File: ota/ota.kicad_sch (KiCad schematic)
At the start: 19 parts, among them J3 Conn_01x04_Pin, J4 Conn_01x04_Pin, Q1 BC856BDW1, Q2 BC846BDW1, Q3 BC846BDW1, Q4 BC856BDW1, Q5 BC846BDW1, Q8 BC846BDW1, Q9 BC856BDW1

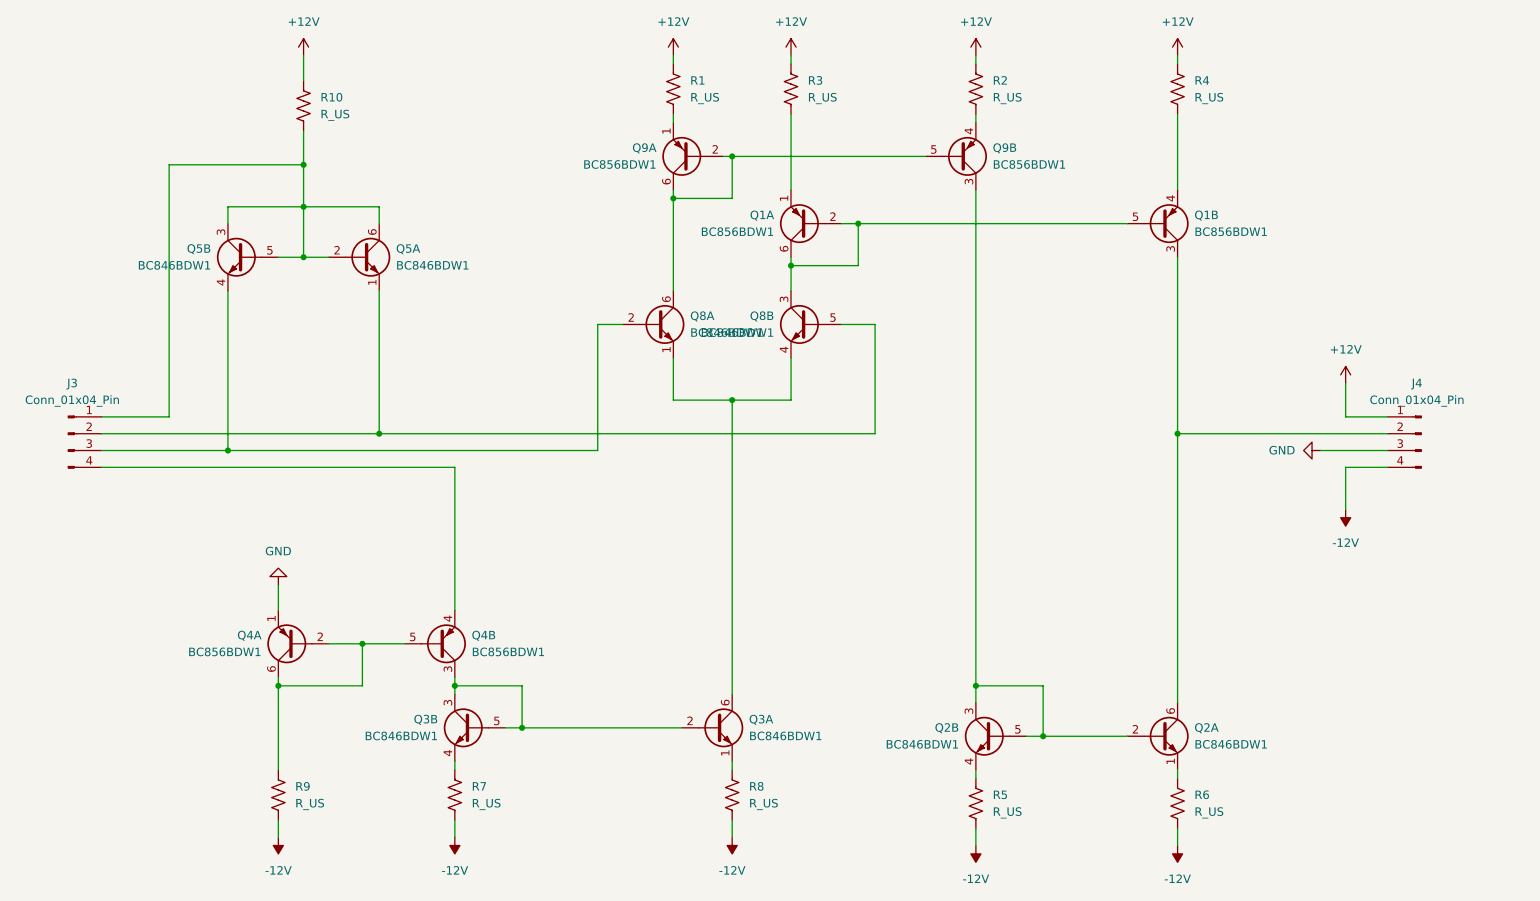
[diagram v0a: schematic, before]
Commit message: v1
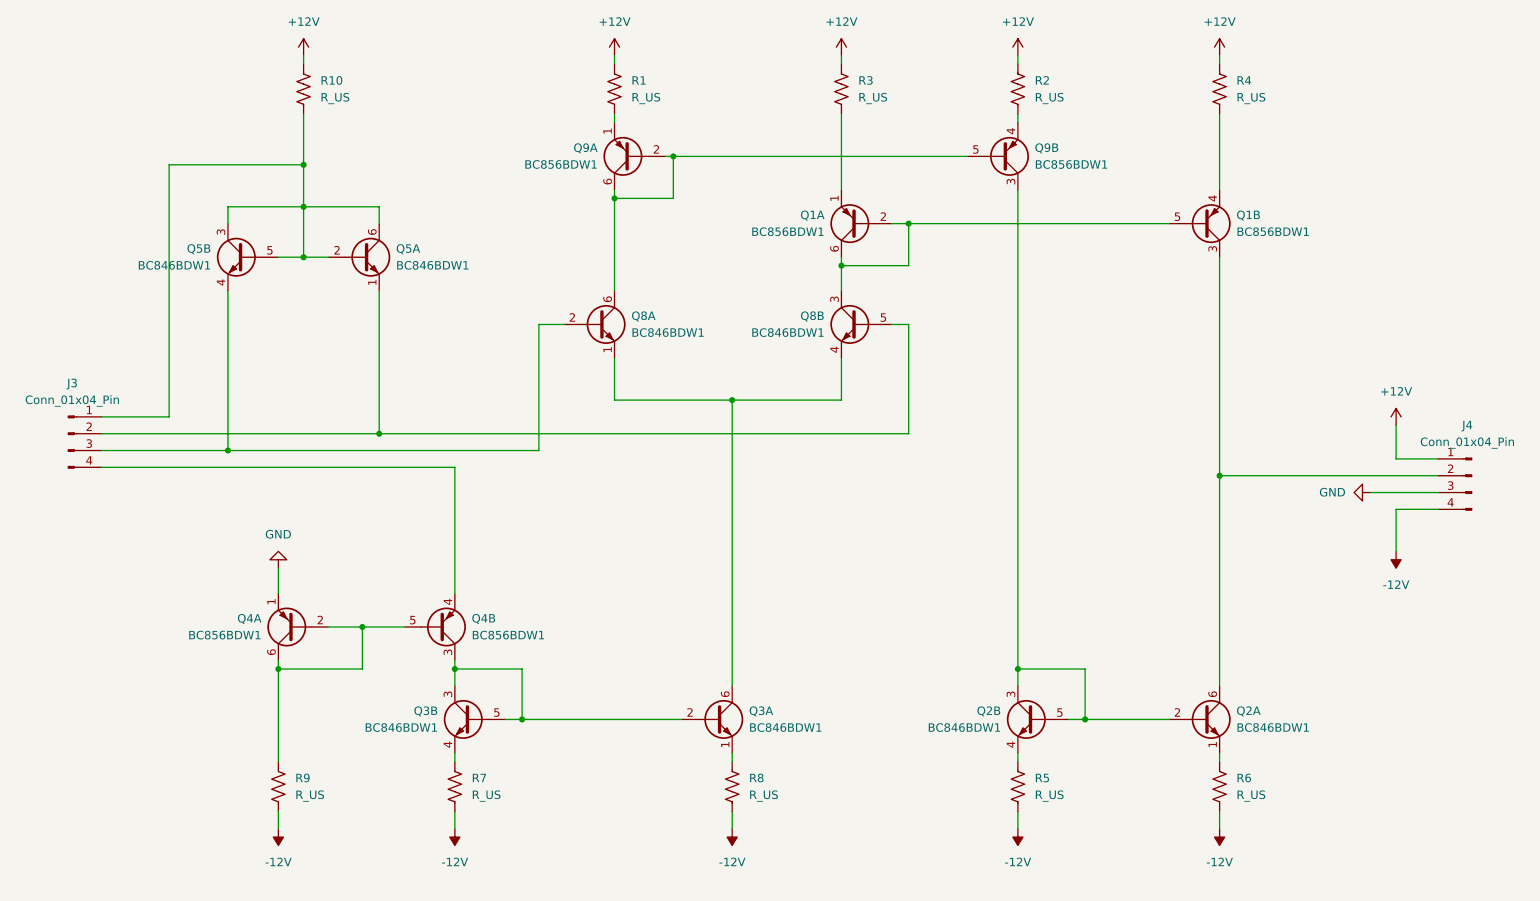
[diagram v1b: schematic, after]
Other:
- moved on the sheet: J4, Q1A, Q1B, Q2A, Q2B, Q3A, Q3B, Q4A, Q4B, Q8A, Q8B, Q9A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
